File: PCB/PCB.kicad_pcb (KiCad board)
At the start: 2 copper layers, 100 x 53 mm, 51 parts, among them J1 USB_C_Receptacle_USB2.0_16P, Q1 NMOS, SW1 RESET, SW2 Button, U1 RP2040, U2 W25Q32JVSS, U4 NCP1117-3.3_SOT223, Y1 12 MHz

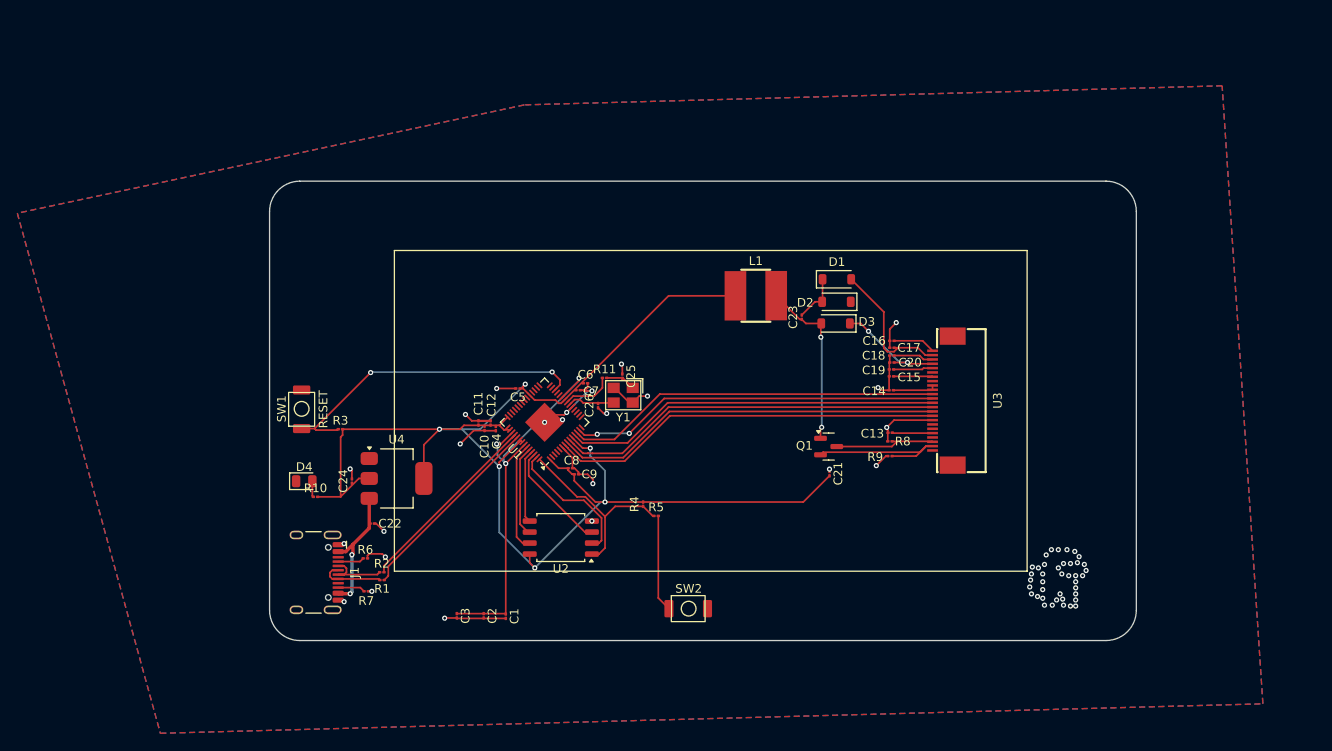
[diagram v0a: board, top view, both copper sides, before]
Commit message: potato
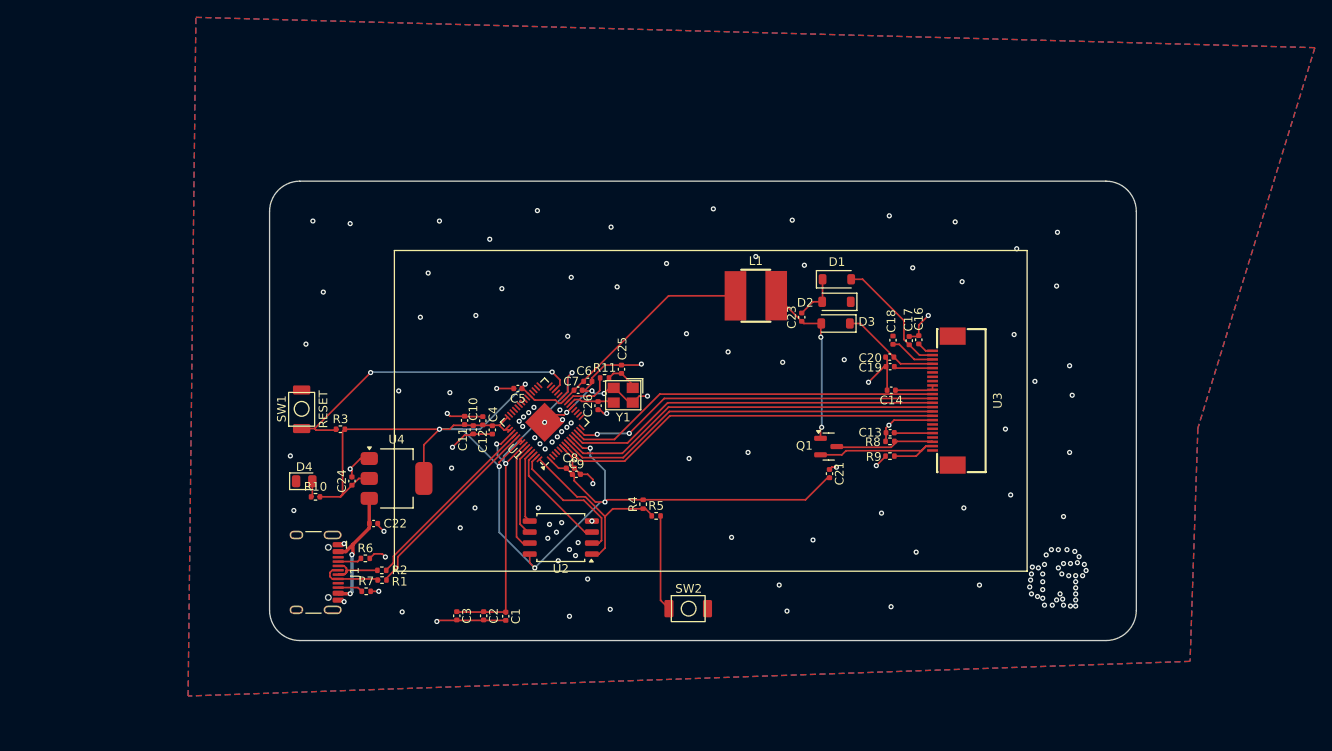
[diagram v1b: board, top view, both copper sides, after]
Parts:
- removed C15: 1uF, Capacitor_SMD:C_01005_0402Metric
- C1, C10, C11, C12, C13, C14, C16, C17, C18, C19, C2, C20, C21, C22, C23, C24, C25, C26, C3, C4, C5, C6, C7, C8, C9: footprint Capacitor_SMD:C_01005_0402Metric -> Capacitor_SMD:C_0402_1005Metric
- R1, R10, R11, R2, R3, R4, R5, R6, R7, R8, R9: footprint Resistor_SMD:R_01005_0402Metric -> Resistor_SMD:R_0402_1005Metric
- moved C16 3.10 mm to (144.9, 68.3), turned to 90 degrees
- moved C17 2.16 mm to (143.8, 68.4), turned to 90 degrees
- moved C18 1.78 mm to (141.9, 68.3), turned to 90 degrees
- moved C11 1.63 mm to (92.5, 77.6)
- moved C10 1.31 mm to (93.5, 78.7)
- moved C12 0.93 mm to (94.6, 77.6)
- moved C25 0.81 mm to (110.6, 71.7)
- moved C20 0.67 mm to (141.6, 70.3)
- moved C4 0.43 mm to (95.7, 78.7)
- moved C19 0.35 mm to (141.6, 71.4)
- moved C6 0.35 mm to (106.7, 73.1)
- moved R2 0.22 mm to (83.0, 94.9)
- moved C22 0.15 mm to (82.0, 89.5)
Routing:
- net BS: track 66.3 -> 81.7 mm, vias 64 -> 149
- net Net-(U3-VDD): track 4.51 -> 0.00 mm
- net VCOM: track 4.92 -> 1.92 mm
- net VGL: track 16.3 -> 14.3 mm
- net VGH: track 13.0 -> 11.5 mm, vias 2 -> 0
- net Net-(U3-VSL): track 4.63 -> 5.29 mm
- net +1V1: track 47.8 -> 48.4 mm
- net RESE: track 11.9 -> 11.4 mm
